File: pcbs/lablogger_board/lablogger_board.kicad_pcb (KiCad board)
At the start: 2 copper layers, 72 x 44 mm, 41 parts, among them J1 RJ45, J2 Conn_01x07, J3 Conn_01x12, J4 PINHD-1X4, P1 24V / 5A, Q1 220mA / 50V, Q2 220mA / 50V, Q3 220mA / 50V, Q4 220mA / 50V, U1 8-28V in / 5V 5W out, U2 Particle2 / Boron

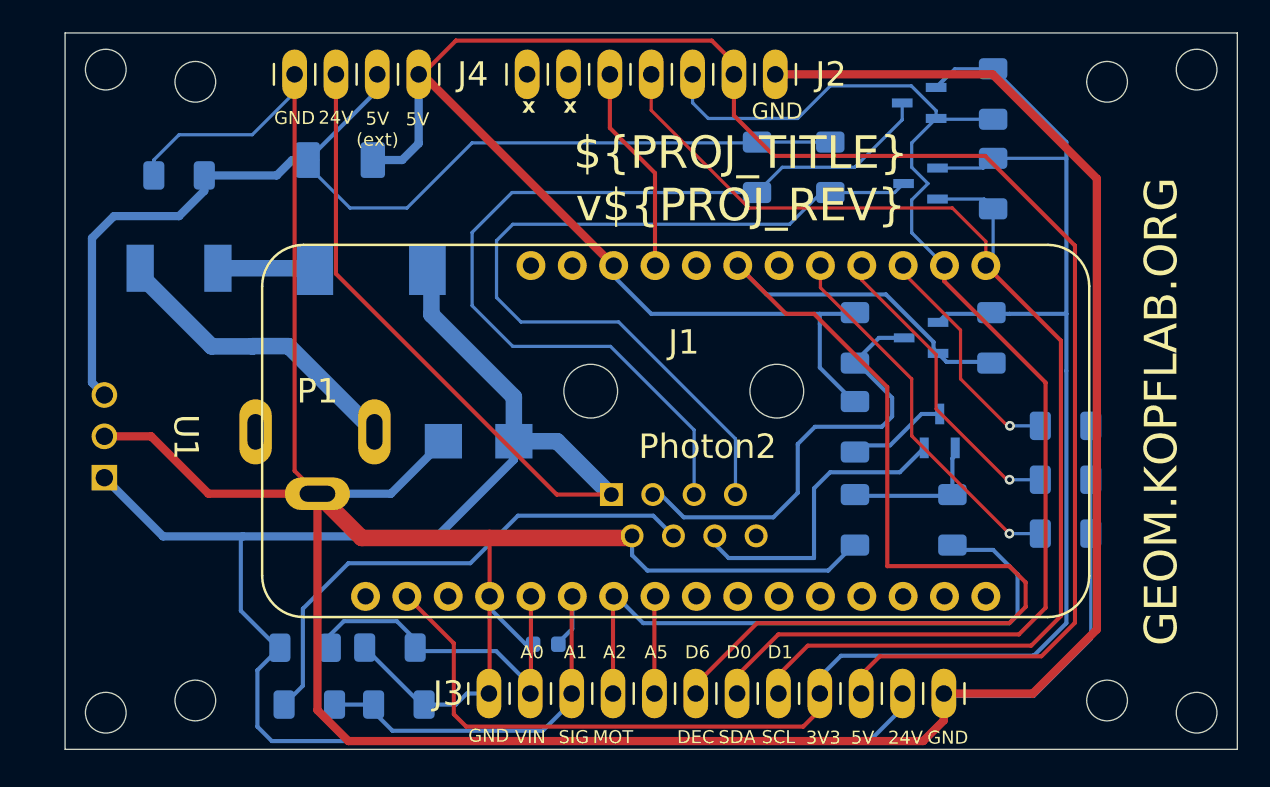
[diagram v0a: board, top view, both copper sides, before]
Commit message: lablogger first version
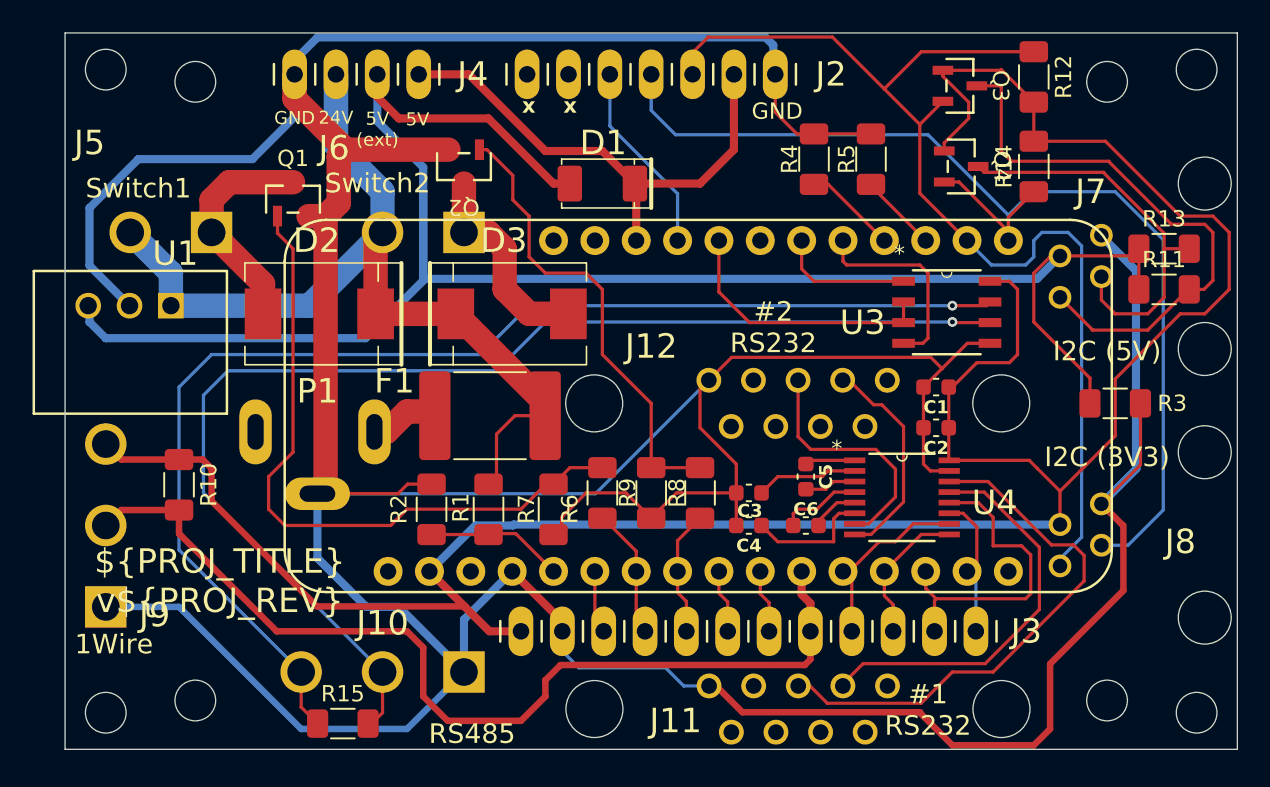
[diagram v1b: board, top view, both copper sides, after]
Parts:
- removed J1: RJ45, footprints:RJ45_A-2014-2-4-N-T-R
- removed R18: 10kΩ, footprints:R_1206
- removed the R4 at (115.0, 121.0)
- removed the R5 at (148.5, 109.7)
- added C2: 100nF, footprints:C_0603, F.Cu at (153.5, 104.0)
- added C3: 100nF, footprints:C_0603, F.Cu at (142.0, 108.0)
- added C4: 100nF, footprints:C_0603, F.Cu at (142.0, 110.0)
- added C5: 100nF, footprints:C_0603, F.Cu at (145.5, 107.0)
- added C6: 100nF, footprints:C_0603, F.Cu at (145.5, 110.0)
- added J10: 5mm, footprints:TERMINAL_BLOCK_1x03_5mm_vertical, B.Cu at (124.5, 119.0)
- added J11: DB9, footprints:DB9_male, B.Cu at (150.5, 119.9)
- added J12: DB9, footprints:DB9_male, B.Cu at (150.5, 101.1)
- added J5: 5mm, footprints:TERMINAL_BLOCK_1x02_5mm_vertical, B.Cu at (109.0, 92.0)
- added J6: 5mm, footprints:TERMINAL_BLOCK_1x02_5mm_vertical, B.Cu at (124.5, 92.0)
- added J7: RJ11, footprints:RJ11_MOLEX_955032641, B.Cu at (163.7, 92.2)
- added J8: RJ11, footprints:RJ11_MOLEX_955032641, B.Cu at (163.7, 108.7)
- added J9: 5mm, footprints:TERMINAL_BLOCK_1x03_5mm_vertical, B.Cu at (102.5, 115.0)
- added R15: 120Ω, footprints:R_1206, F.Cu at (117.1, 122.2)
- added U3: RS485 Transceiver, footprints:8-SOIC, F.Cu at (154.2, 96.9)
- added U4: RS232 Transceiver, footprints:TSSOP16_MXL, F.Cu at (151.4, 108.3)
- C1: value 10nF -> 100nF; moved to F.Cu
- D1: value 3A/60V/750mV -> 1A/40V/500mV; footprint footprints:D_DO-214AB_SMC -> footprints:D_DO-214AC_SMA; moved to F.Cu
- D2: value 1A/40V/500mV -> 3A/60V/750mV; footprint footprints:D_DO-214AC_SMA -> footprints:D_DO-214AB_SMC; moved to F.Cu
- D3: value 40V -> 3A/60V/750mV; footprint footprints:D_DO-214AA_SMB -> footprints:D_DO-214AB_SMC; moved to F.Cu
- F1: value 33V/750mA/1.5A -> 24V/2.6A; footprint footprints:Fuse_1812 -> footprints:Fuse_2920_7451; moved to F.Cu
- Q1, Q2: value 220mA / 50V -> 5.7A / 30V; moved to F.Cu
- Q3, Q4, R1, R11, R12, R13, R14, R2, R7, R9, U1: moved to F.Cu
- R10: value 10kΩ -> 4.7kΩ; moved to F.Cu
- R3: value 100kΩ -> 10kΩ; moved to F.Cu
- R4: renamed from R17; moved to F.Cu
- R5: renamed from R16; moved to F.Cu
- R6: value 150Ω -> 100Ω; moved to F.Cu
- R8: value 1kΩ -> 100Ω; moved to F.Cu
- moved R10 50.7 mm to (107.0, 107.5), turned to -90 degrees
- moved R3 47.7 mm to (164.5, 102.5)
- moved Q1 42.2 mm to (114.0, 90.0), turned to 0 degrees
- moved R7 30.8 mm to (130.0, 109.0), turned to -90 degrees
- moved Q2 30.0 mm to (124.5, 88.0), turned to 180 degrees
- moved C1 28.7 mm to (153.5, 101.5)
- moved R11 26.1 mm to (167.5, 95.5), turned to 0 degrees
- moved R4 25.0 mm to (146.0, 87.5), turned to -90 degrees
- moved R6 21.6 mm to (133.0, 108.0)
- moved F1 21.1 mm to (126.1, 103.3)
- moved R13 21.1 mm to (167.5, 93.0), turned to 0 degrees
- moved R5 20.3 mm to (149.5, 87.5), turned to -90 degrees
- moved R9 15.7 mm to (136.0, 108.0)
- moved D1 15.0 mm to (133.0, 89.0)
- moved R1 14.1 mm to (126.0, 109.0), turned to -90 degrees
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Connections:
- net /A2-MOTOR renamed /A2-Switch1
- C1 pad 1: /A1-SIGNAL -> +3V3
- D1 pad 1: +24V -> +5V
- D1 pad 2: Net-(D1-A) -> +5Vout
- D2 pad 1: +5V -> +24V
- D2 pad 2: +5Vout -> Net-(D2-A)
- D3 pad 2: GND -> Net-(D3-A)
- F1 pad 1: Net-(D1-A) -> +24V
- J3 pad 1: GND -> +3V3
- J3 pad 10: +5V -> /D16-RX
- J3 pad 11: +24V -> /RX
- J3 pad 12: GND -> /TX
- J3 pad 2: /A0-VIN -> GND
- J3 pad 3: /A1-SIGNAL -> /A1
- J3 pad 5: /A5 -> /A5-Switch2
- J3 pad 6: /D6-DECO -> /S4
- J3 pad 7: /D1-SCL -> /S3
- J3 pad 8: /D0-SDA -> /D17-1Wire
- J3 pad 9: +3V3 -> /D15-TX
- Q1 pad 2: /5V-SPEED -> GND
- Q1 pad 3: Net-(Q1-D) -> Net-(D2-A)
- Q2 pad 1: +3V3 -> Net-(Q2-G)
- Q2 pad 2: /D6-DECO -> GND
- Q2 pad 3: /5V-DECO -> Net-(D3-A)
- R10 pad 1: /D6-DECO -> +3V3
- R10 pad 2: +3V3 -> /D17-1Wire
- R3 pad 1: /A1-SIGNAL -> +5Vout
- R7 pad 1: +5Vout -> Net-(Q1-G)
- R8 pad 1: +5V -> /A5-Switch2
- R8 pad 2: Net-(Q1-D) -> Net-(Q2-G)
- R9 pad 1: +5V -> Net-(Q2-G)
- R9 pad 2: /5V-DECO -> GND
- U2 pad 11: /SCK -> /D17-1Wire
- U2 pad 12: /MOSI -> /D15-TX
- U2 pad 13: /MISO -> /D16-RX
- U2 pad 21: /D4 -> /D4-TX
- U2 pad 22: /D5 -> /D5-RX
- U2 pad 23: /D6-DECO -> /D6
- U2 pad 24: /D7 -> /D7-RTS
- U2 pad 6: /A1-SIGNAL -> /A1
- U2 pad 8: /A5 -> /A5-Switch2
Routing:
- net +5V: track 134.2 -> 31.3 mm
- net +24V: track 139.4 -> 56.7 mm
- net /RS485-B: track 0.00 -> 76.2 mm, vias 0 -> 1
- net /RS485-A: track 0.00 -> 75.4 mm, vias 0 -> 1
- net /D6-DECO: track 74.8 -> 0.00 mm
- net /D17-1Wire: track 0.00 -> 59.4 mm
- net GND: track 262.5 -> 316.9 mm
- net +5Vout: track 67.7 -> 116.8 mm
- net +3V3: track 106.4 -> 150.0 mm
- net /TO-RS232 #1: track 0.00 -> 32.9 mm
- net Net-(Q1-G): track 8.96 -> 41.4 mm
- net /SIGNAL: track 32.0 -> 0.00 mm
- net /A2-Switch1: track 39.2 -> 8.06 mm
- net Net-(Q2-G): track 0.00 -> 28.6 mm
- net /5V-DECO: track 27.6 -> 0.00 mm
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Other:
- board text added: "#1 RS232"
- board text added: "#2 RS232"
- board text added: "1Wire"
- board text added: "I2C (3V3)"
- board text added: "I2C (5V)"
- board text added: "RS485"
- board text added: "Switch1"
- board text added: "Switch2"
- board text removed: "3V3"
- board text removed: "A0"
- board text removed: "A1"
- board text removed: "A2"
- board text removed: "A5"
- board text removed: "D0"
- board text removed: "D1"
- board text removed: "D6"
- board text removed: "DEC"
- board text removed: "GEOM.KOPFLAB.ORG"
- board text removed: "MOT"
- board text removed: "Photon2"
- board text removed: "SCL"
- board text removed: "SDA"
- board text removed: "SIG"
- board text removed: "VIN"
